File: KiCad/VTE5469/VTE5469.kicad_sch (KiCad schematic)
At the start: 34 parts, among them J1 Power, J2 JRD-100 (UHF RFID), J3 Program, J4 Display, Q1 BD138, Q3 BC547, SW1 Switch, SW2 Reset, SW3 Mode, U1 AMS1117-3.3, U2 ESP-12F, U3 MQ-2, U4 Vibration, U5 XD-58C, U6 DHT11

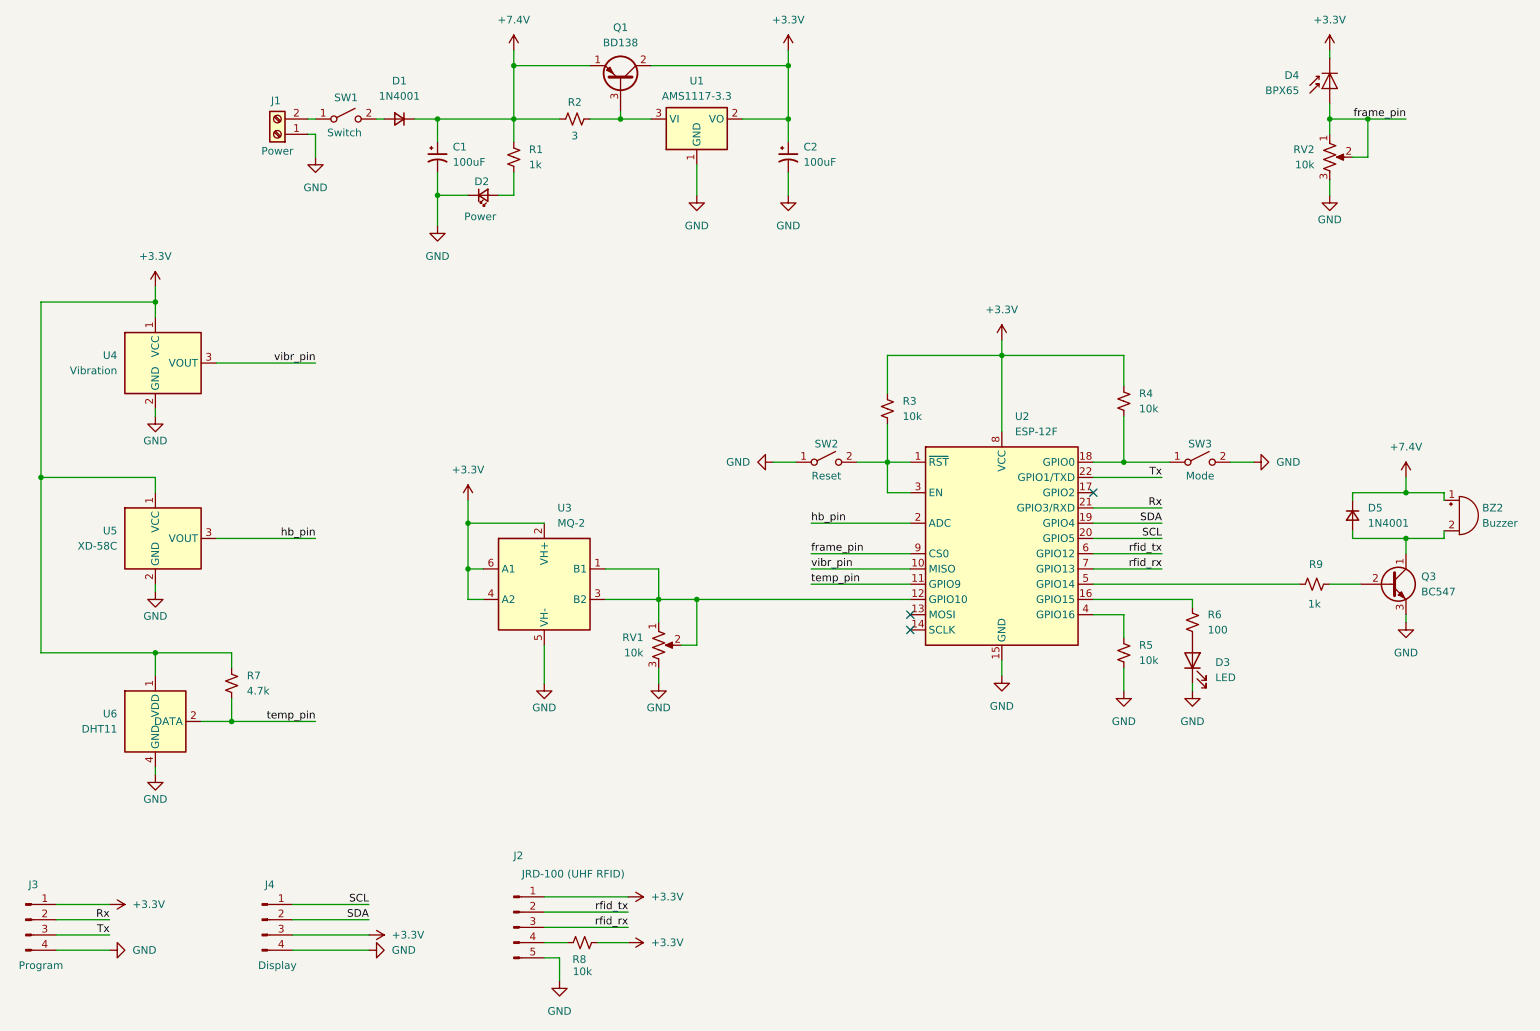
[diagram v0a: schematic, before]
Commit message: latest updated
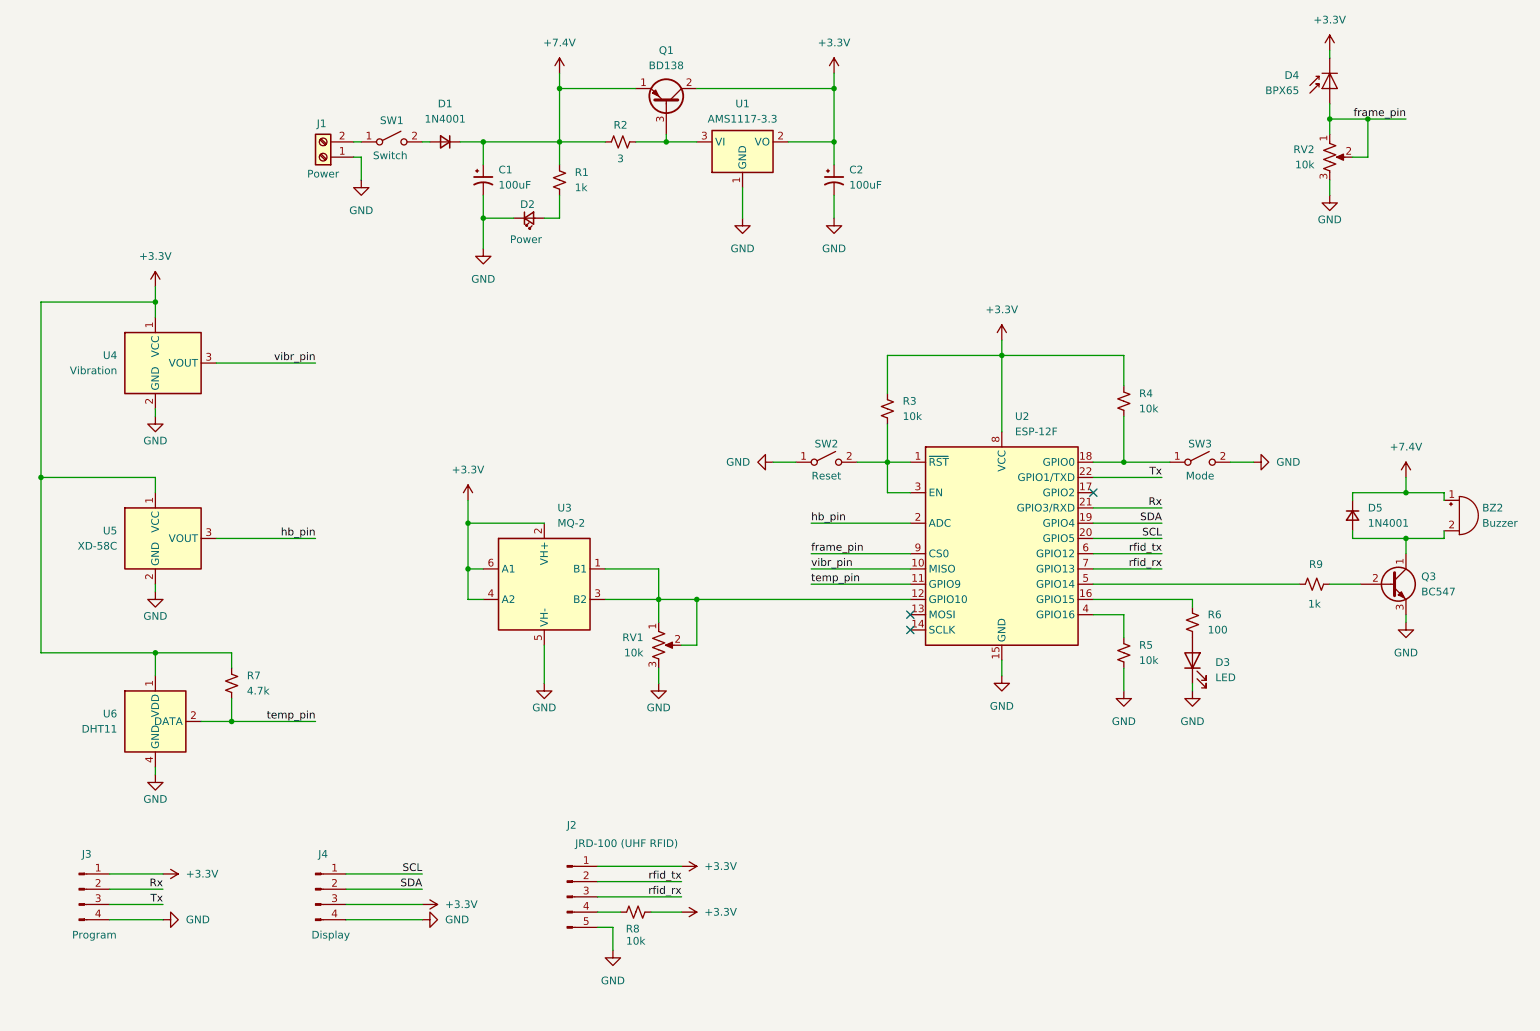
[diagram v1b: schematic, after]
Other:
- moved on the sheet: C1, C2, D1, D2, J1, J2, J3, J4, Q1, R1, R2, R8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
